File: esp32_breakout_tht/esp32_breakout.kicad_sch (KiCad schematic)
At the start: 16 parts, among them J1 AUX1, J10 UART1, J11 ADC3, J12 SPI1, J13 ADC4, J14 DAC1, J15 DAC2, J16 SPI2, J2 AUX2, J4 ADC1, J5 ADC2, J6 I2C1, J7 I2C2, J8 I2C3, J9 I2C4, U1 ESP32-DEVKITC-32D

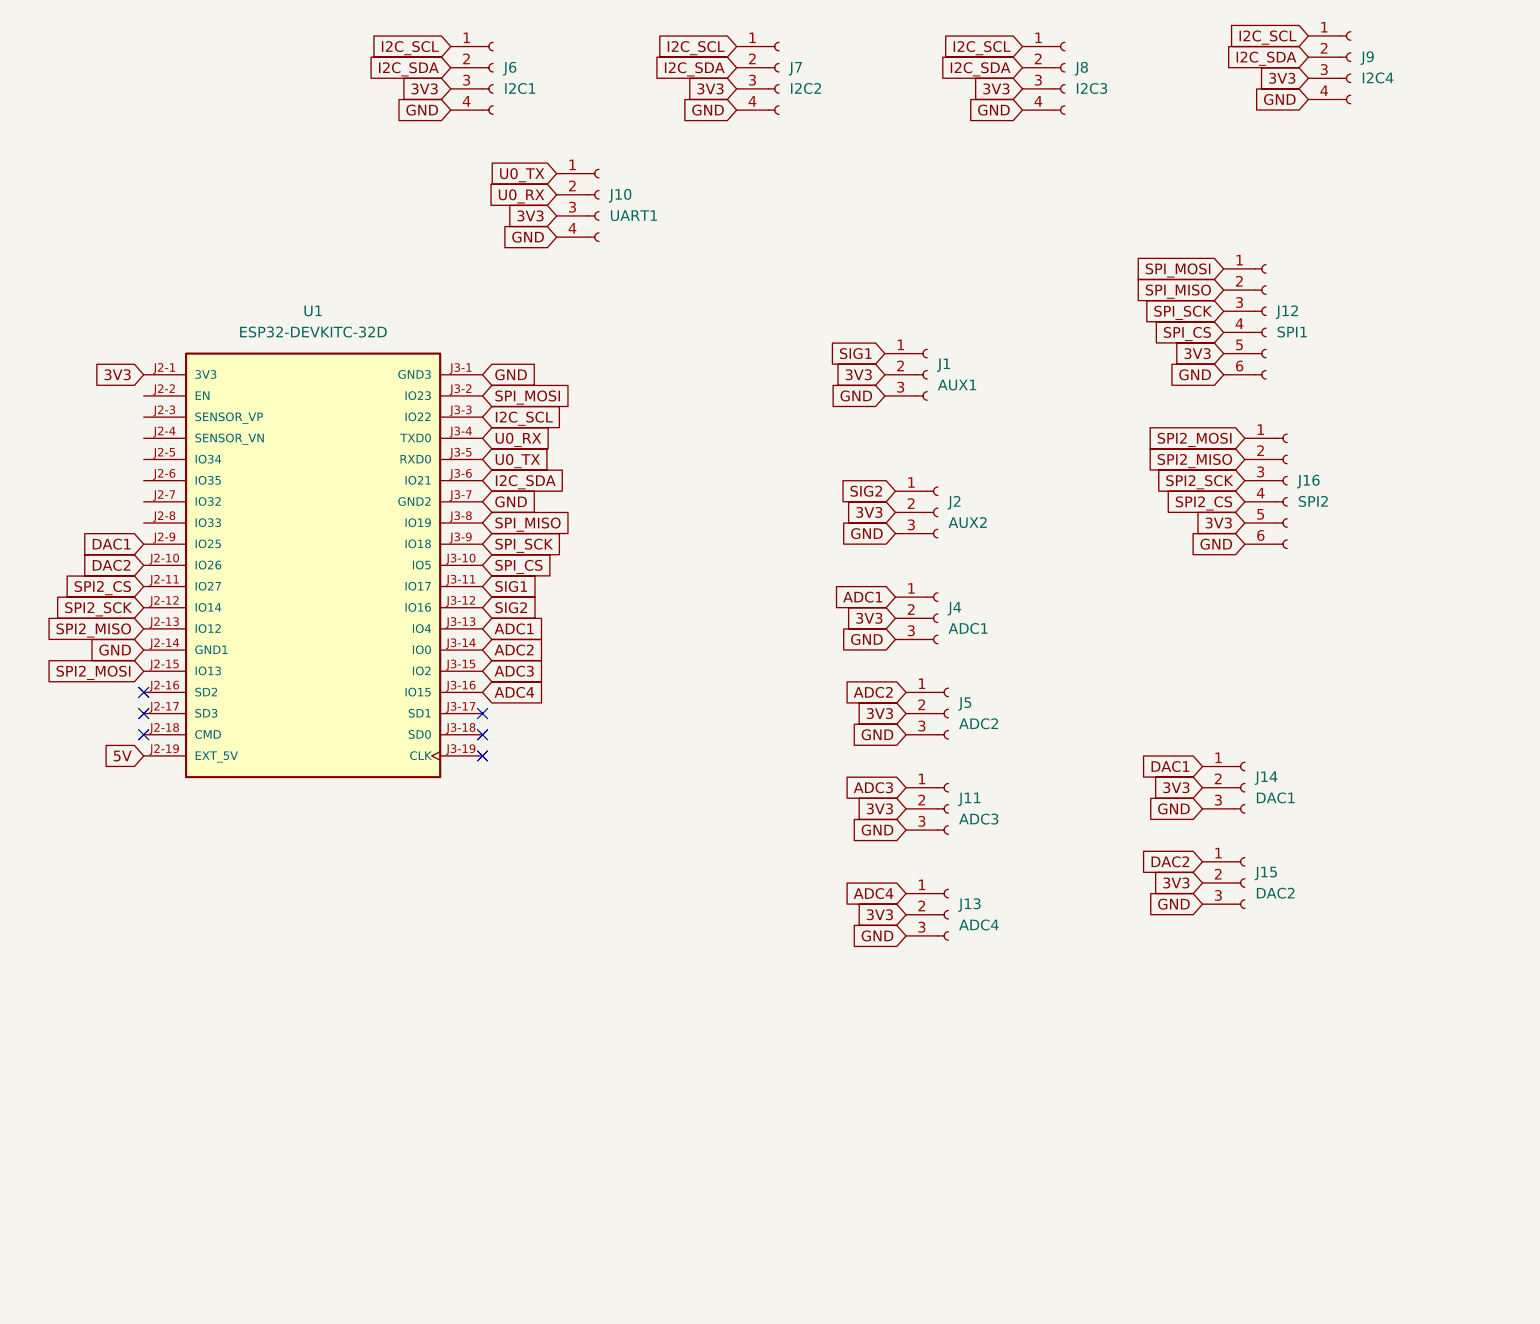
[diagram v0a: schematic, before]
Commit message: made shield style boards
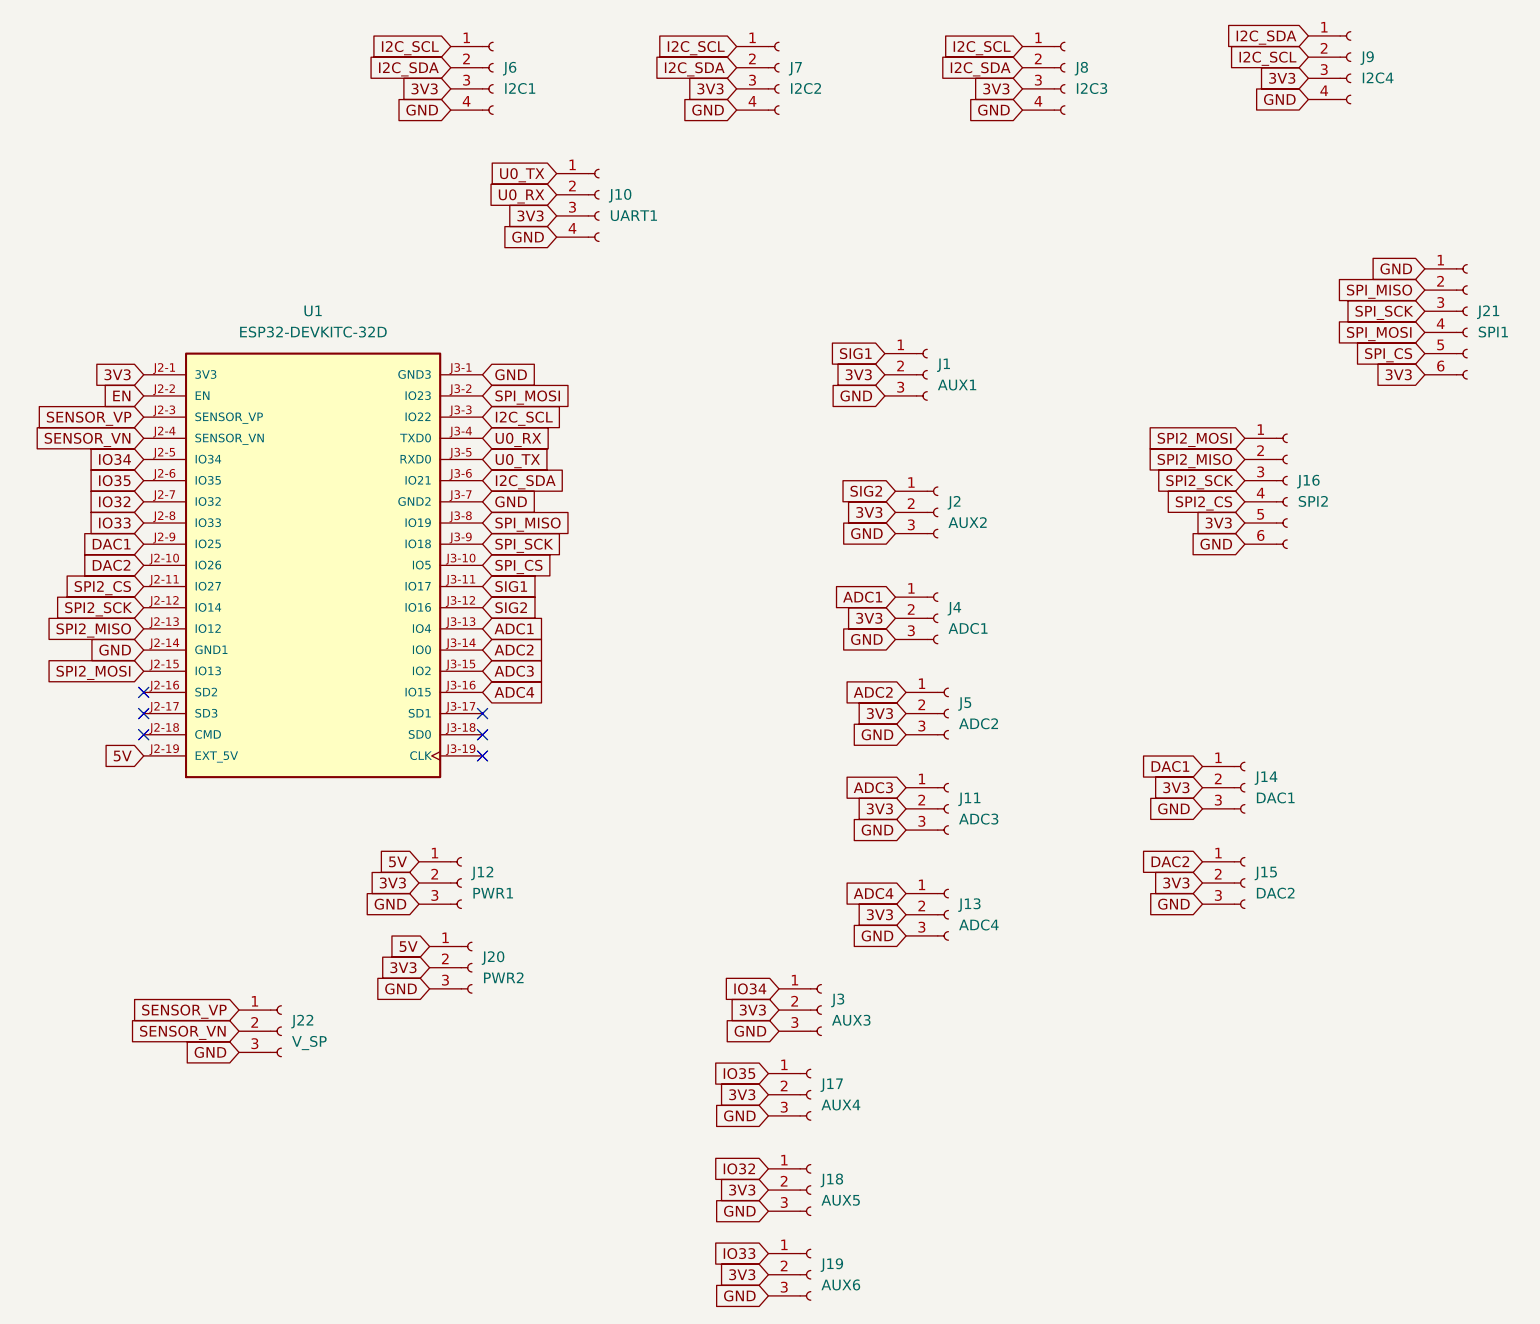
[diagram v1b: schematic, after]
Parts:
- removed J12: SPI1, Connector_PinSocket_2.00mm:PinSocket_1x06_P2.00mm_Vertical_SMD_Pin1Left, symbol Connector:Conn_01x06_Socket
- added J12: PWR1, Connector_PinHeader_2.54mm:PinHeader_1x03_P2.54mm_Vertical, symbol Connector:Conn_01x03_Socket
- added J17: AUX4, Connector_PinHeader_2.54mm:PinHeader_1x03_P2.54mm_Vertical, symbol Connector:Conn_01x03_Socket
- added J18: AUX5, Connector_PinHeader_2.54mm:PinHeader_1x03_P2.54mm_Vertical, symbol Connector:Conn_01x03_Socket
- added J19: AUX6, Connector_PinHeader_2.54mm:PinHeader_1x03_P2.54mm_Vertical, symbol Connector:Conn_01x03_Socket
- added J20: PWR2, Connector_PinHeader_2.54mm:PinHeader_1x03_P2.54mm_Vertical, symbol Connector:Conn_01x03_Socket
- added J21: SPI1, Connector_PinHeader_2.54mm:PinHeader_1x06_P2.54mm_Vertical, symbol Connector:Conn_01x06_Socket
- added J22: V_SP, Connector_PinHeader_2.54mm:PinHeader_1x03_P2.54mm_Vertical, symbol Connector:Conn_01x03_Socket
- added J3: AUX3, Connector_PinHeader_2.54mm:PinHeader_1x03_P2.54mm_Vertical, symbol Connector:Conn_01x03_Socket
- J1, J11, J13, J14, J15, J2, J4, J5: footprint Connector_PinSocket_2.00mm:PinSocket_1x03_P2.00mm_Vertical_SMD_Pin1Left -> Connector_PinHeader_2.54mm:PinHeader_1x03_P2.54mm_Vertical
- J10, J6, J7, J8, J9: footprint Connector_PinSocket_2.00mm:PinSocket_1x04_P2.00mm_Vertical_SMD_Pin1Left -> Connector_PinHeader_2.54mm:PinHeader_1x04_P2.54mm_Vertical
- J16: footprint Connector_PinSocket_2.00mm:PinSocket_1x06_P2.00mm_Vertical_SMD_Pin1Left -> Connector_PinHeader_2.54mm:PinHeader_1x06_P2.54mm_Vertical
- U1: footprint ESP32-DEVKITC-32D:MODULE_ESP32-DEVKITC-32D -> ESP32-DEVKITC-32D:MODULE_ESP32-DEVKITC-32D-THT
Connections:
- net 3V3: now also J12.2 (Pin_2), J17.2 (Pin_2), J18.2 (Pin_2), J19.2 (Pin_2), J20.2 (Pin_2), J21.6 (Pin_6), J3.2 (Pin_2)
- net 5V: now also J12.1 (Pin_1), J20.1 (Pin_1)
- net GND: now also J12.3 (Pin_3), J17.3 (Pin_3), J18.3 (Pin_3), J19.3 (Pin_3), J20.3 (Pin_3), J21.1 (Pin_1), J22.3 (Pin_3), J3.3 (Pin_3)
- net I2C_SCL: now also J9.2 (Pin_2); no longer J9.1 (Pin_1)
- net I2C_SDA: now also J9.1 (Pin_1); no longer J9.2 (Pin_2)
- net SPI_CS: now also J21.5 (Pin_5)
- net SPI_MISO: now also J21.2 (Pin_2)
- net SPI_MOSI: now also J21.4 (Pin_4)
- net SPI_SCK: now also J21.3 (Pin_3)
- net EN: now reaches U1.J2-2 (EN)
- net SENSOR_VP: now reaches U1.J2-3 (SENSOR_VP)
- net SENSOR_VP: now also J22.1 (Pin_1)
- net SENSOR_VN: now reaches U1.J2-4 (SENSOR_VN)
- net SENSOR_VN: now also J22.2 (Pin_2)
- net IO34: now reaches U1.J2-5 (IO34)
- net IO34: now also J3.1 (Pin_1)
- net IO35: now reaches U1.J2-6 (IO35)
- net IO35: now also J17.1 (Pin_1)
- net IO32: now reaches U1.J2-7 (IO32)
- net IO32: now also J18.1 (Pin_1)
- net IO33: now reaches U1.J2-8 (IO33)
- net IO33: now also J19.1 (Pin_1)
